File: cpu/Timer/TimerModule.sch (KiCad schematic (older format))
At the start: 17 parts, among them J1 Interconnect, U1 LM555, U2 74LS00, U3 74LS00, U4 74LS365

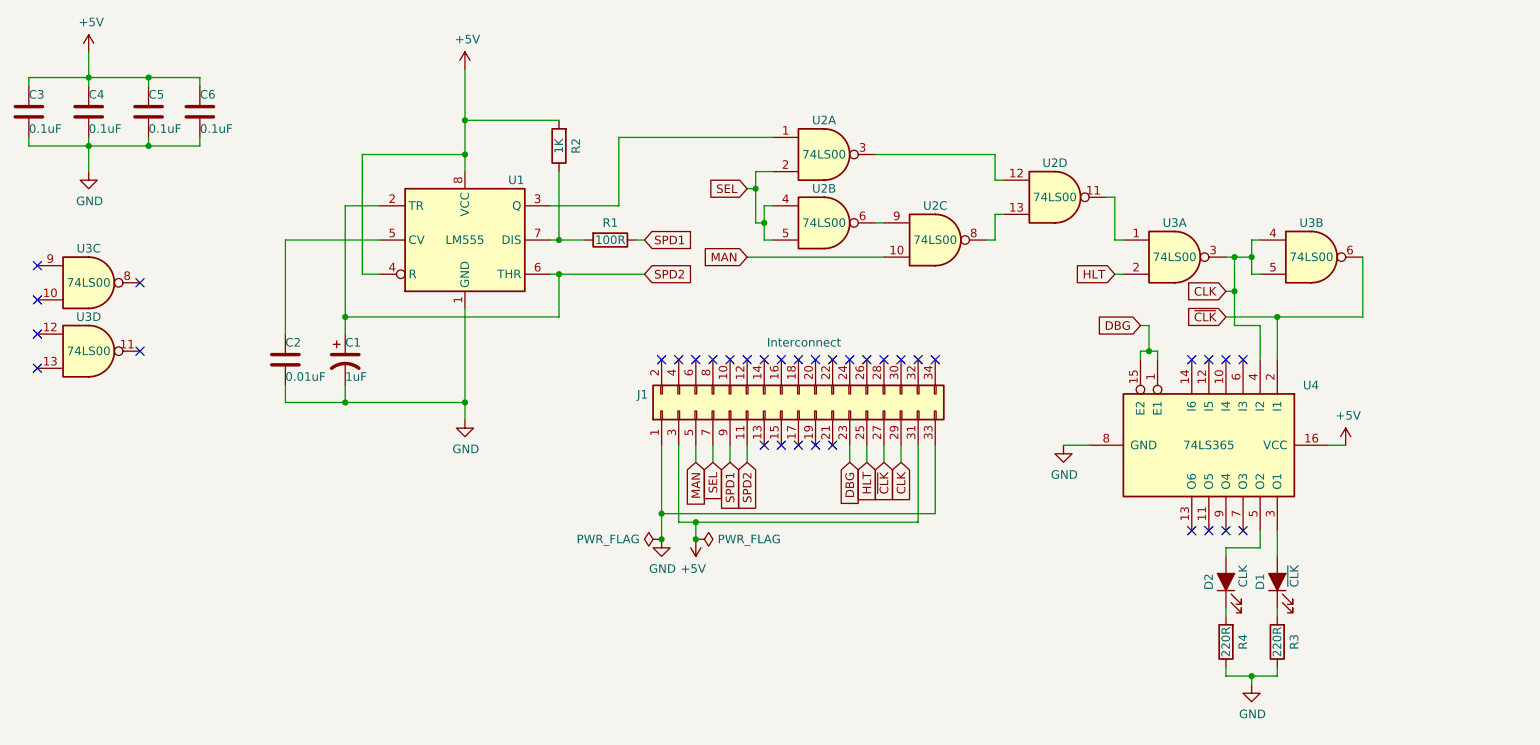
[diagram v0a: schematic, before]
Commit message: Lots of changes
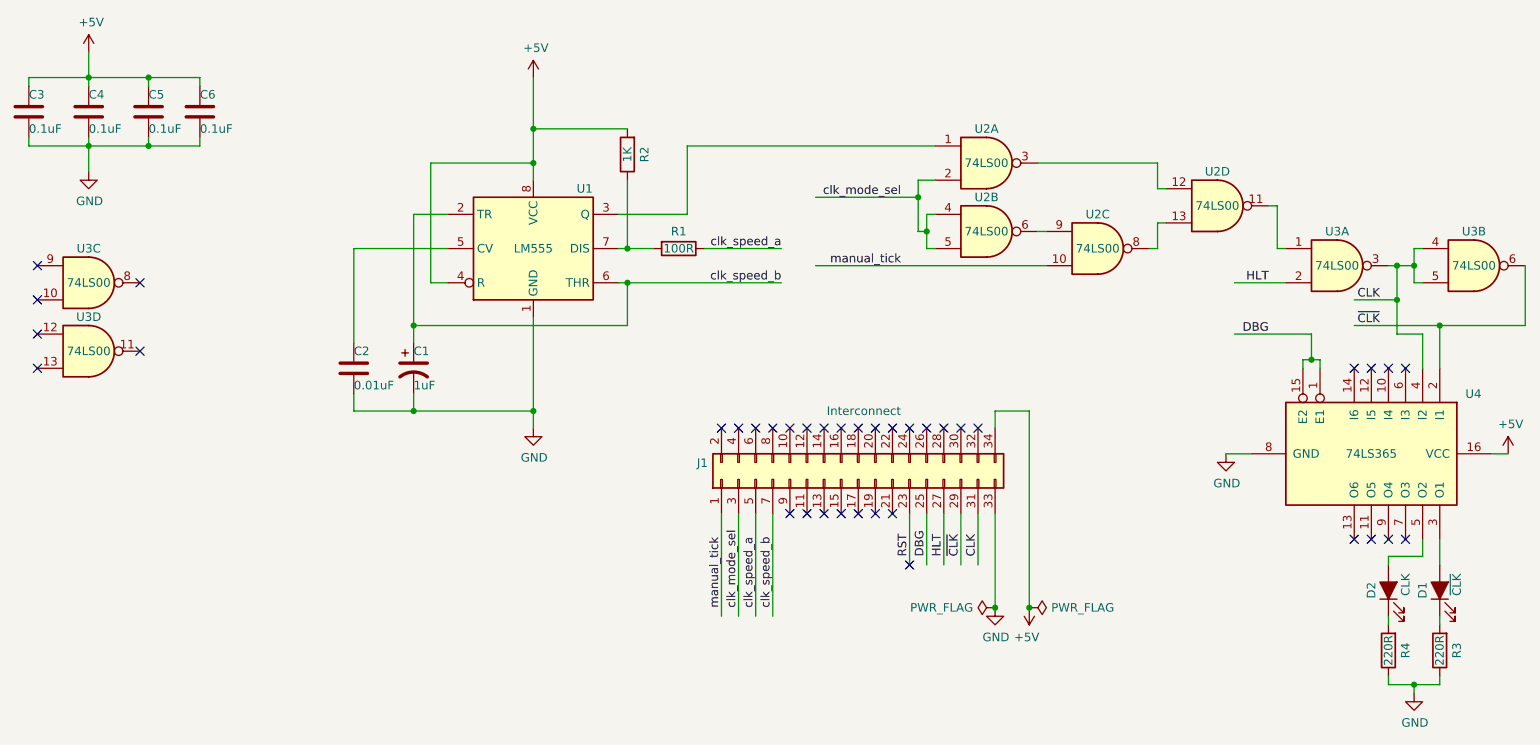
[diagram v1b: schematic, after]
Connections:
- net labels added: RST, clk_mode_sel, clk_speed_a, clk_speed_b, manual_tick
- net labels removed: MAN, SEL, SPD1, SPD2
- wire segments 117 -> 113
- no-connect marks 36 -> 38
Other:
- moved on the sheet: C1, C2, D1, D2, J1, R1, R2, R3, R4, U1, U2A, U2B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
